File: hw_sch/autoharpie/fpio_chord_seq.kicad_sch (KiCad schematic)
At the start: 60 parts, among them SW100 SW_Push_45deg, SW101 SW_Push_45deg, SW102 SW_Push_45deg, SW103 SW_Push_45deg, SW104 SW_Push_45deg, SW105 SW_Push_45deg, SW106 SW_Push_45deg, SW107 SW_Push_45deg, SW108 SW_Push_45deg, SW109 SW_Push_45deg, SW110 SW_Push_45deg, SW111 SW_Push_45deg, SW112 SW_Push_45deg, SW113 SW_Push_45deg, SW114 SW_Push_45deg, SW115 SW_Push_45deg, SW116 SW_Push_45deg, SW117 SW_Push_45deg, SW118 SW_Push_45deg, SW119 SW_Push_45deg, SW120 SW_Push_45deg, SW121 SW_Push_45deg, SW122 SW_Push_45deg, SW123 SW_Push_45deg, SW124 SW_Push_45deg, SW125 SW_Push_45deg, SW126 SW_Push_45deg, SW127 SW_Push_45deg, SW128 SW_Push_45deg, SW129 SW_Push_45deg, SW130 SW_Push_45deg, SW131 SW_Push_45deg, SW132 SW_Push_45deg, SW133 SW_Push_45deg, SW134 SW_Push_45deg, SW135 SW_Push_45deg, SW136 SW_Push_45deg, SW77 SW_Push_45deg, SW78 SW_Push_45deg, SW79 SW_Push_45deg, SW80 SW_Push_45deg, SW81 SW_Push_45deg, SW82 SW_Push_45deg, SW83 SW_Push_45deg, SW84 SW_Push_45deg, SW85 SW_Push_45deg, SW86 SW_Push_45deg, SW87 SW_Push_45deg, SW88 SW_Push_45deg, SW89 SW_Push_45deg, SW90 SW_Push_45deg, SW91 SW_Push_45deg, SW92 SW_Push_45deg, SW93 SW_Push_45deg, SW94 SW_Push_45deg, SW95 SW_Push_45deg, SW96 SW_Push_45deg, SW97 SW_Push_45deg, SW98 SW_Push_45deg, SW99 SW_Push_45deg

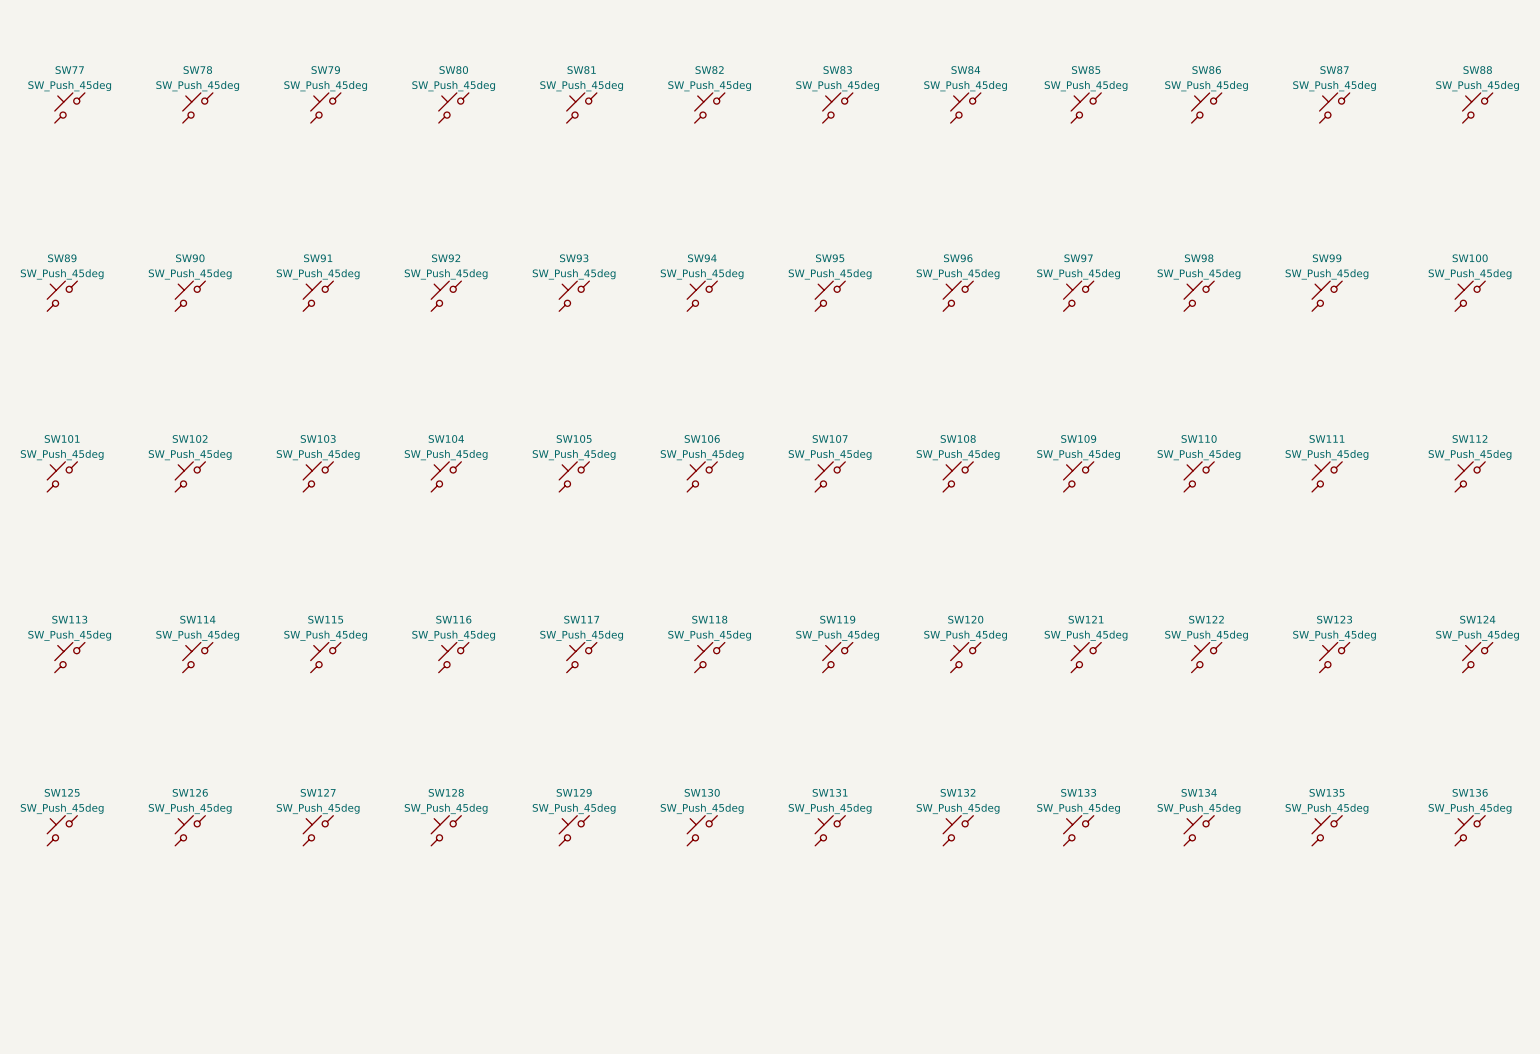
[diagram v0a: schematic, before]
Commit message: isolated ground
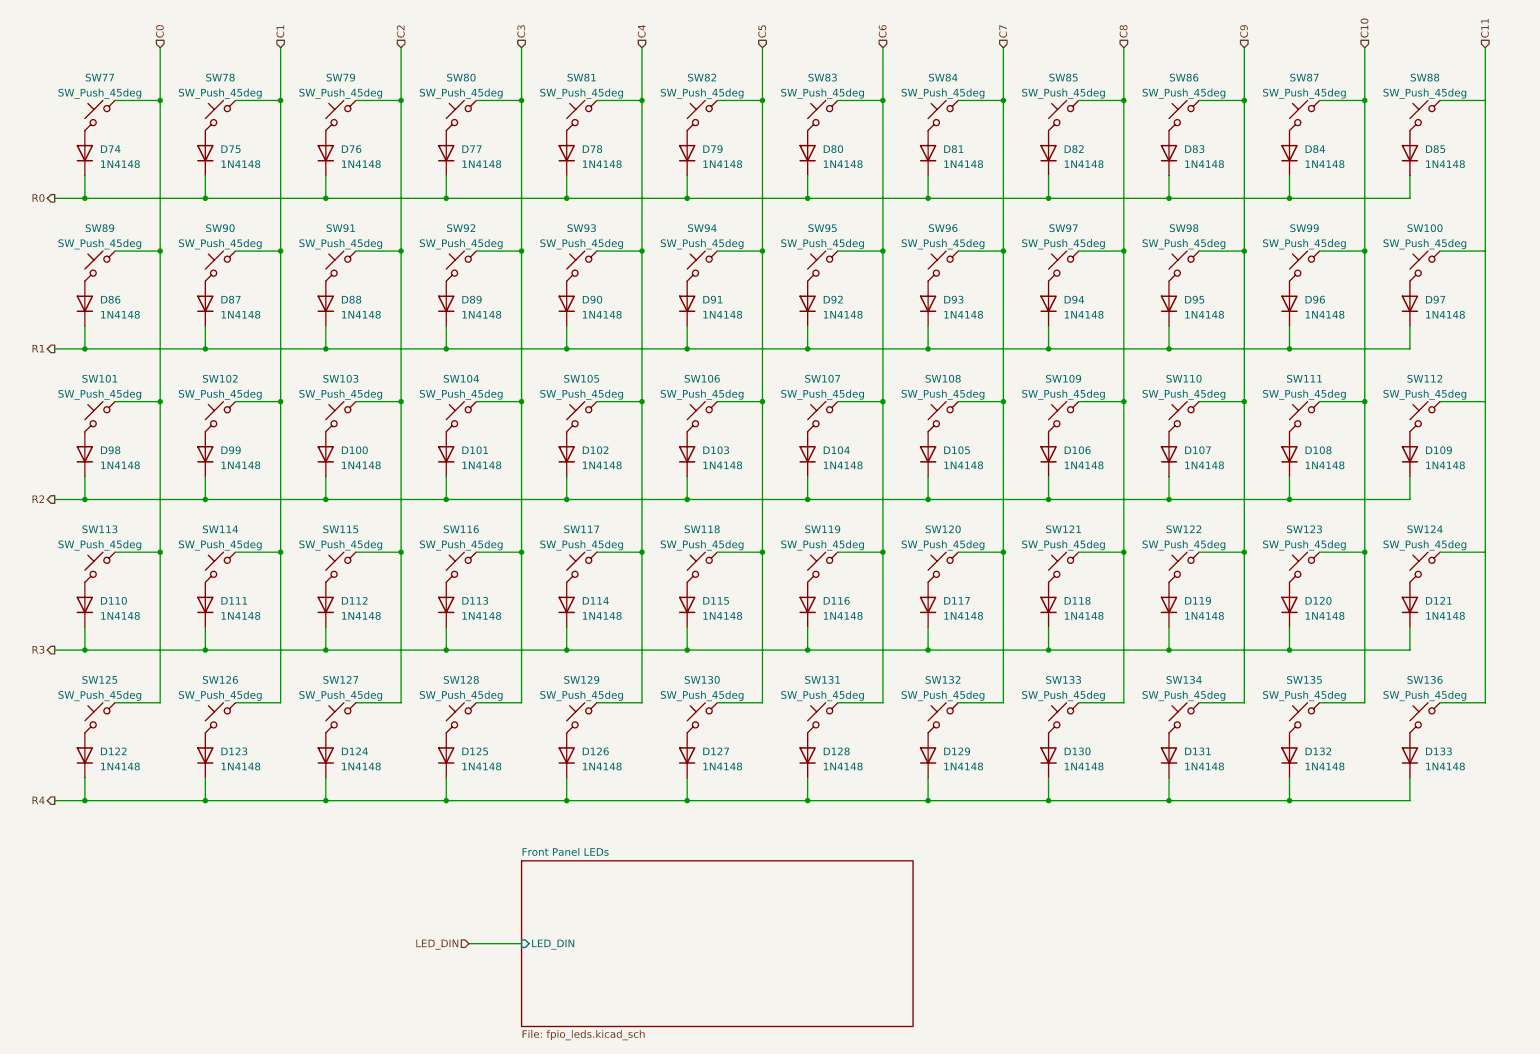
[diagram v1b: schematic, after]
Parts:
- added D100, D101, D102, D103, D104, D105, D106, D107, D108, D109, D110, D111, D112, D113, D114, D115, D116, D117, D118, D119, D120, D121, D122, D123, D124, D125, D126, D127, D128, D129, D130, D131, D132, D133, D74, D75, D76, D77, D78, D79, D80, D81, D82, D83, D84, D85, D86, D87, D88, D89, D90, D91, D92, D93, D94, D95, D96, D97, D98, D99: 1N4148, symbol Device:D
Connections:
- net at SW100.2: now also D97.2 (A)
- net C9: now reaches SW134.1
- net C9: now also SW110.1, SW122.1, SW86.1, SW98.1
- net at SW134.2: now also D131.2 (A)
- net C1: now reaches SW126.1
- net C1: now also SW102.1, SW114.1, SW78.1, SW90.1
- net at SW126.2: now also D123.2 (A)
- net C2: now reaches SW103.1
- net C2: now also SW115.1, SW127.1, SW79.1, SW91.1
- net at SW103.2: now also D100.2 (A)
- net C3: now reaches SW92.1
- net C3: now also SW104.1, SW116.1, SW128.1, SW80.1
- net at SW92.2: now also D89.2 (A)
- net C0: now reaches SW77.1
- net C0: now also SW101.1, SW113.1, SW125.1, SW89.1
- net at SW77.2: now also D74.2 (A)
- net C5: now reaches SW106.1
- net C5: now also SW118.1, SW130.1, SW82.1, SW94.1
- net at SW106.2: now also D103.2 (A)
- net at SW125.2: now also D122.2 (A)
- net at SW90.2: now also D87.2 (A)
- net C8: now reaches SW133.1
- net C8: now also SW109.1, SW121.1, SW85.1, SW97.1
- net at SW133.2: now also D130.2 (A)
- net at SW110.2: now also D107.2 (A)
- net at SW98.2: now also D95.2 (A)
- net C6: now reaches SW131.1
- net C6: now also SW107.1, SW119.1, SW83.1, SW95.1
- net at SW131.2: now also D128.2 (A)
- net C7: now reaches SW120.1
- net C7: now also SW108.1, SW132.1, SW84.1, SW96.1
- net at SW120.2: now also D117.2 (A)
- net at SW85.2: now also D82.2 (A)
- net at SW102.2: now also D99.2 (A)
- net at SW108.2: now also D105.2 (A)
- net at SW96.2: now also D93.2 (A)
- net at SW107.2: now also D104.2 (A)
- net C10: now reaches SW135.1
- net C10: now also SW111.1, SW123.1, SW87.1, SW99.1
- net at SW135.2: now also D132.2 (A)
- net at SW86.2: now also D83.2 (A)
- net at SW116.2: now also D113.2 (A)
- net at SW113.2: now also D110.2 (A)
- net at SW83.2: now also D80.2 (A)
- net C4: now reaches SW81.1
- net C4: now also SW105.1, SW117.1, SW129.1, SW93.1
- net at SW81.2: now also D78.2 (A)
- net at SW94.2: now also D91.2 (A)
- net at SW79.2: now also D76.2 (A)
- net at SW122.2: now also D119.2 (A)
- net at SW111.2: now also D108.2 (A)
- net at SW115.2: now also D112.2 (A)
- net at SW130.2: now also D127.2 (A)
- net at SW82.2: now also D79.2 (A)
- net at SW127.2: now also D124.2 (A)
- net at SW93.2: now also D90.2 (A)
- net at SW95.2: now also D92.2 (A)
- net at SW101.2: now also D98.2 (A)
- net at SW117.2: now also D114.2 (A)
- net at SW99.2: now also D96.2 (A)
- net at SW124.2: now also D121.2 (A)
- net at SW114.2: now also D111.2 (A)
- net at SW121.2: now also D118.2 (A)
- net at SW118.2: now also D115.2 (A)
- net at SW129.2: now also D126.2 (A)
- net at SW87.2: now also D84.2 (A)
- net at SW84.2: now also D81.2 (A)
- net at SW91.2: now also D88.2 (A)
- net at SW109.2: now also D106.2 (A)
- net at SW112.2: now also D109.2 (A)
- net at SW80.2: now also D77.2 (A)
- net at SW88.2: now also D85.2 (A)
- net at SW105.2: now also D102.2 (A)
- net at SW132.2: now also D129.2 (A)
- net at SW97.2: now also D94.2 (A)
- net at SW123.2: now also D120.2 (A)
- net at SW78.2: now also D75.2 (A)
- net at SW128.2: now also D125.2 (A)
- net at SW89.2: now also D86.2 (A)
- net at SW104.2: now also D101.2 (A)
- net at SW119.2: now also D116.2 (A)
- net at SW136.2: now also D133.2 (A)
- new net R0: D74.1 (K), D75.1 (K), D76.1 (K), D77.1 (K), D78.1 (K), D79.1 (K), D80.1 (K), D81.1 (K), D82.1 (K), D83.1 (K), D84.1 (K), D85.1 (K)
- new net R1: D86.1 (K), D87.1 (K), D88.1 (K), D89.1 (K), D90.1 (K), D91.1 (K), D92.1 (K), D93.1 (K), D94.1 (K), D95.1 (K), D96.1 (K), D97.1 (K)
- new net R2: D100.1 (K), D101.1 (K), D102.1 (K), D103.1 (K), D104.1 (K), D105.1 (K), D106.1 (K), D107.1 (K), D108.1 (K), D109.1 (K), D98.1 (K), D99.1 (K)
- new net R3: D110.1 (K), D111.1 (K), D112.1 (K), D113.1 (K), D114.1 (K), D115.1 (K), D116.1 (K), D117.1 (K), D118.1 (K), D119.1 (K), D120.1 (K), D121.1 (K)
- new net R4: D122.1 (K), D123.1 (K), D124.1 (K), D125.1 (K), D126.1 (K), D127.1 (K), D128.1 (K), D129.1 (K), D130.1 (K), D131.1 (K), D132.1 (K), D133.1 (K)
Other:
- added sheet Front Panel LEDs (fpio_leds.kicad_sch)
- moved on the sheet: SW77, SW78, SW79, SW80, SW81, SW82, SW83, SW84, SW85, SW86, SW87, SW88
